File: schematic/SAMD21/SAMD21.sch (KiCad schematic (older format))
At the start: 1 part, among them IC1 ATSAMD21G18A-AU

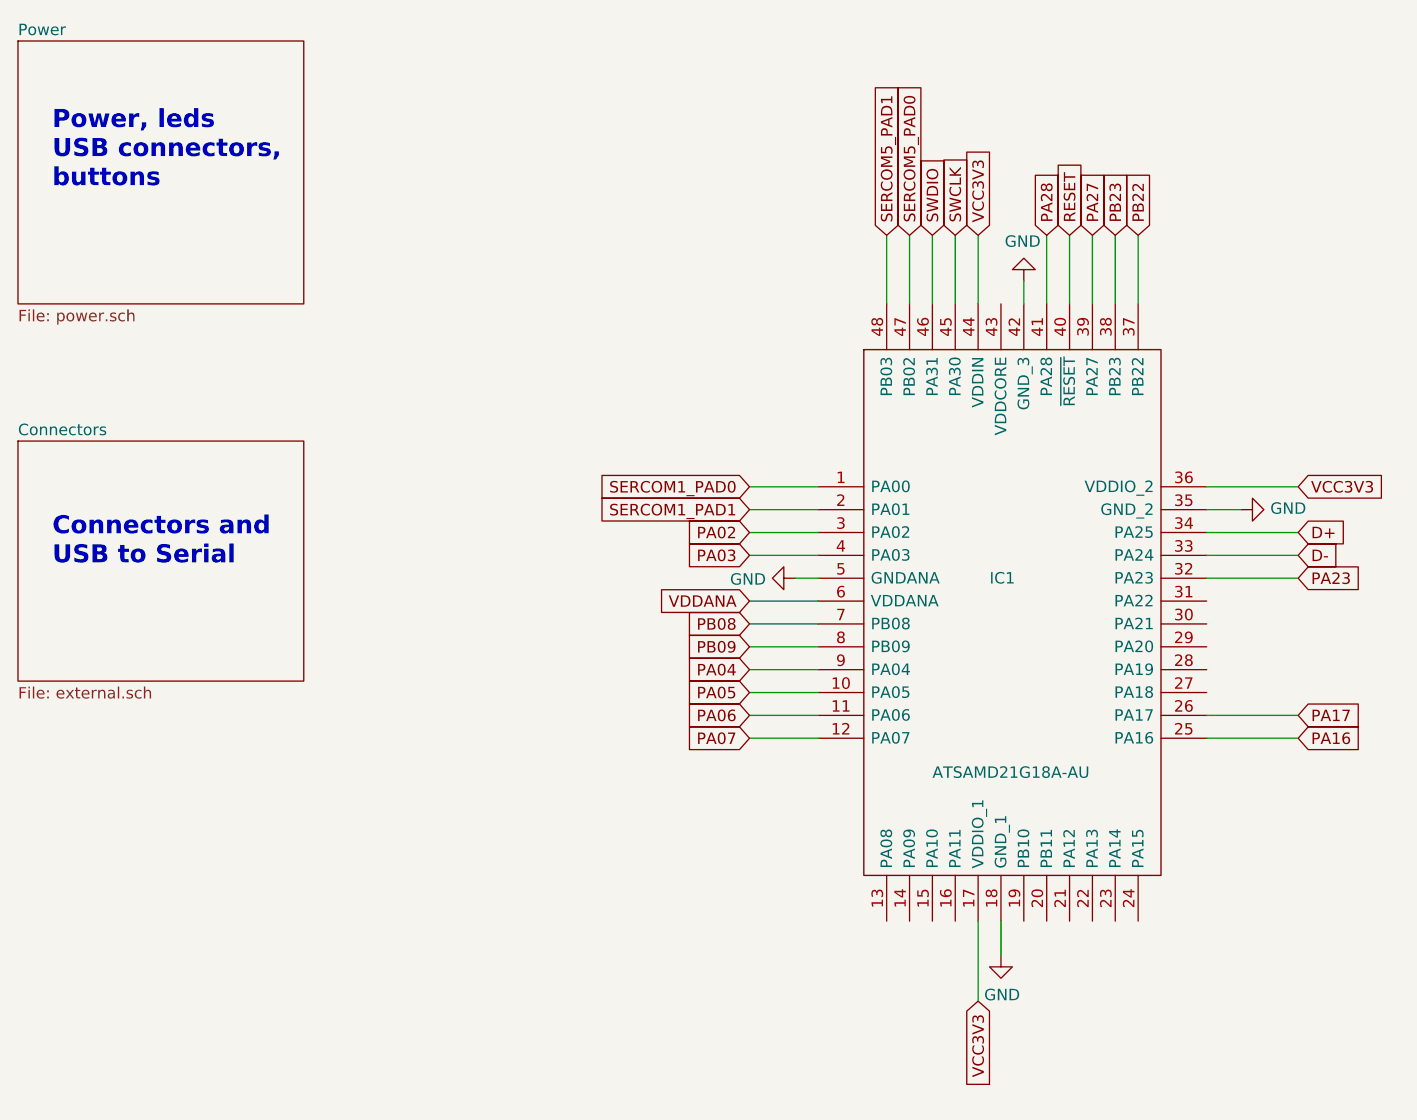
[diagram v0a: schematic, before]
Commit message: Complete schematic
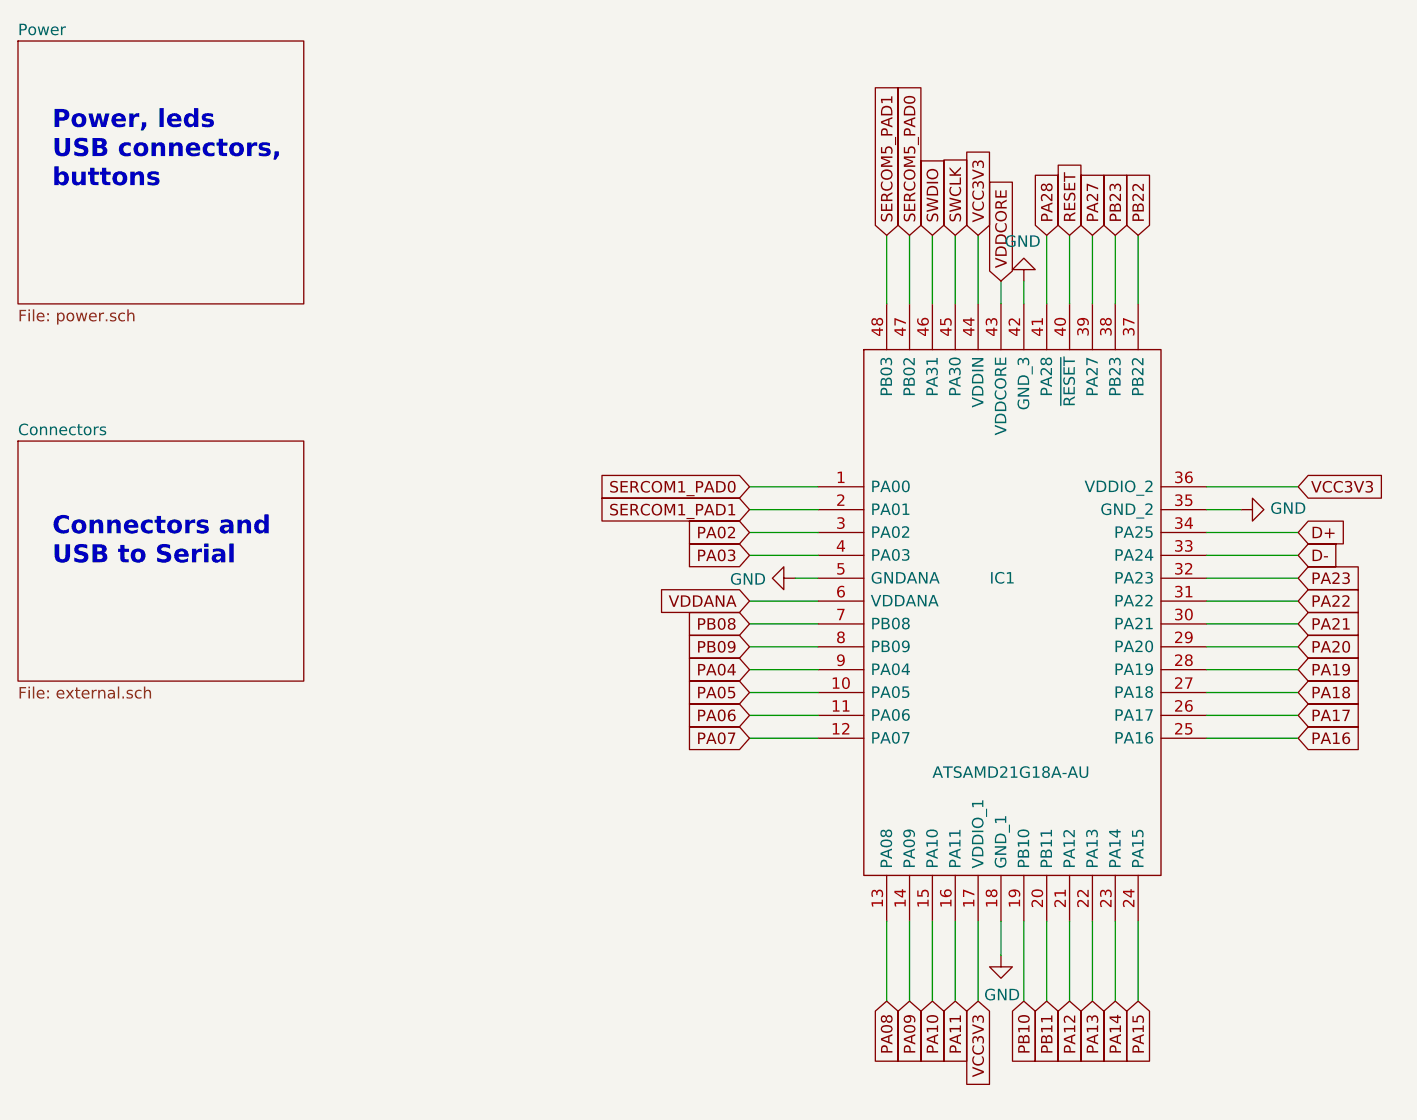
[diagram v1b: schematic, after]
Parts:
- IC1: footprint QFP50P900X900X120-48N -> SamacSys_Parts:QFP50P900X900X120-48N
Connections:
- net PA08: now reaches IC1.13 (PA08)
- net PA09: now reaches IC1.14 (PA09)
- net PA10: now reaches IC1.15 (PA10)
- net PA11: now reaches IC1.16 (PA11)
- net PB10: now reaches IC1.19 (PB10)
- net PB11: now reaches IC1.20 (PB11)
- net PA12: now reaches IC1.21 (PA12)
- net PA13: now reaches IC1.22 (PA13)
- net PA14: now reaches IC1.23 (PA14)
- net PA15: now reaches IC1.24 (PA15)
- net PA18: now reaches IC1.27 (PA18)
- net PA19: now reaches IC1.28 (PA19)
- net PA20: now reaches IC1.29 (PA20)
- net PA21: now reaches IC1.30 (PA21)
- net PA22: now reaches IC1.31 (PA22)
- net VDDCORE: now reaches IC1.43 (VDDCORE)
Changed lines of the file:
@@
 F 0 "IC1" H 5350 2700 50  0000 L CNN
 F 1 "ATSAMD21G18A-AU" H 5100 1850 50  0000 L CNN
-F 2 "QFP50P900X900X120-48N" H 6150 3700 50  0001 L CNN
+F 2 "SamacSys_Parts:QFP50P900X900X120-48N" H 6150 3700 50  0001 L CNN
 F 3 "" H 6150 3600 50  0001 L CNN
 F 4 "ATMEL - ATSAMD21G18A-AU - MCU, 32BIT, CORTEX-M0+, 48MHZ, TQFP-48" H 6150 3500 50  0001 L CNN "Description"
@@
 Wire Wire Line
 	4300 4200 4600 4200
+Text GLabel 4900 5350 3    50   Input ~ 0
+PA08
+Text GLabel 5000 5350 3    50   Input ~ 0
+PA09
+Text GLabel 5100 5350 3    50   Input ~ 0
+PA10
+Text GLabel 5200 5350 3    50   Input ~ 0
+PA11
+Text GLabel 5500 5350 3    50   Input ~ 0
+PB10
+Text GLabel 5600 5350 3    50   Input ~ 0
+PB11
+Text GLabel 5700 5350 3    50   Input ~ 0
+PA12
+Text GLabel 5800 5350 3    50   Input ~ 0
+PA13
+Text GLabel 5900 5350 3    50   Input ~ 0
+PA14
+Text GLabel 6000 5350 3    50   Input ~ 0
+PA15
+Text GLabel 6700 4000 2    50   Input ~ 0
+PA18
+Text GLabel 6700 3900 2    50   Input ~ 0
+PA19
+Text GLabel 6700 3800 2    50   Input ~ 0
+PA20
+Text GLabel 6700 3700 2    50   Input ~ 0
+PA21
+Text GLabel 6700 3600 2    50   Input ~ 0
+PA22
+Wire Wire Line
+	6300 3600 6700 3600
+Wire Wire Line
+	6300 3700 6700 3700
+Wire Wire Line
+	6300 3800 6700 3800
+Wire Wire Line
+	6300 3900 6700 3900
+Wire Wire Line
+	6300 4000 6700 4000
+Wire Wire Line
+	4900 5000 4900 5350
+Wire Wire Line
+	5000 5000 5000 5350
+Wire Wire Line
+	5100 5000 5100 5350
+Wire Wire Line
+	5200 5000 5200 5350
+Wire Wire Line
+	5500 5000 5500 5350
+Wire Wire Line
+	5600 5000 5600 5350
+Wire Wire Line
+	5700 5000 5700 5350
+Wire Wire Line
+	5800 5000 5800 5350
+Wire Wire Line
+	5900 5000 5900 5350
+Wire Wire Line
+	6000 5000 6000 5350
+Text GLabel 5400 2200 1    50   Input ~ 0
+VDDCORE
+Wire Wire Line
+	5400 2300 5400 2200
 $EndSCHEMATC
